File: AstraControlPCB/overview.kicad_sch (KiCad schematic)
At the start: 4 parts

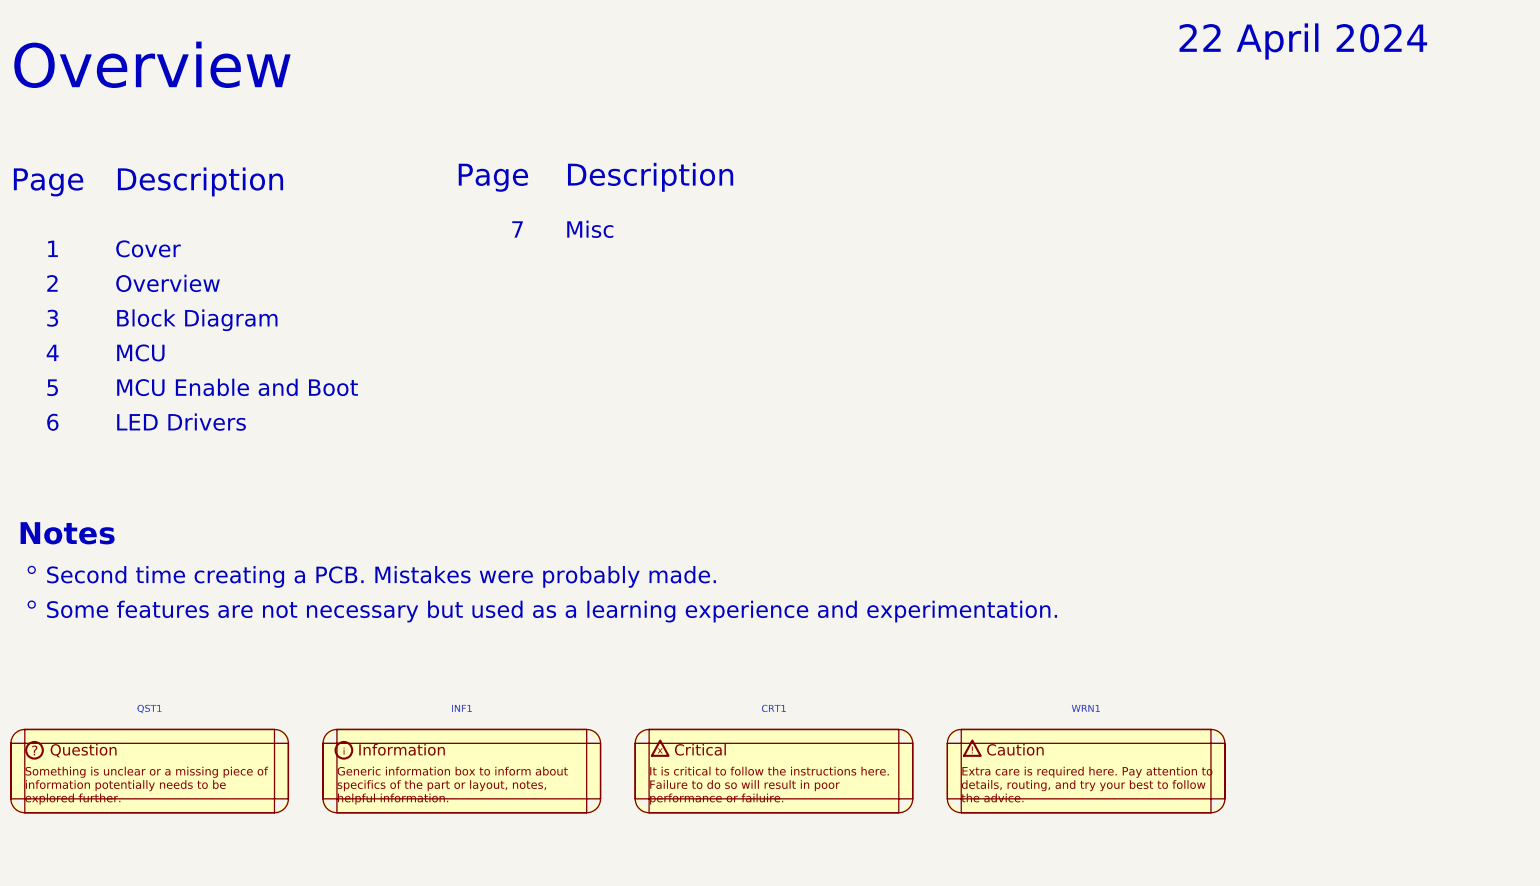
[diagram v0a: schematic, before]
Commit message: update
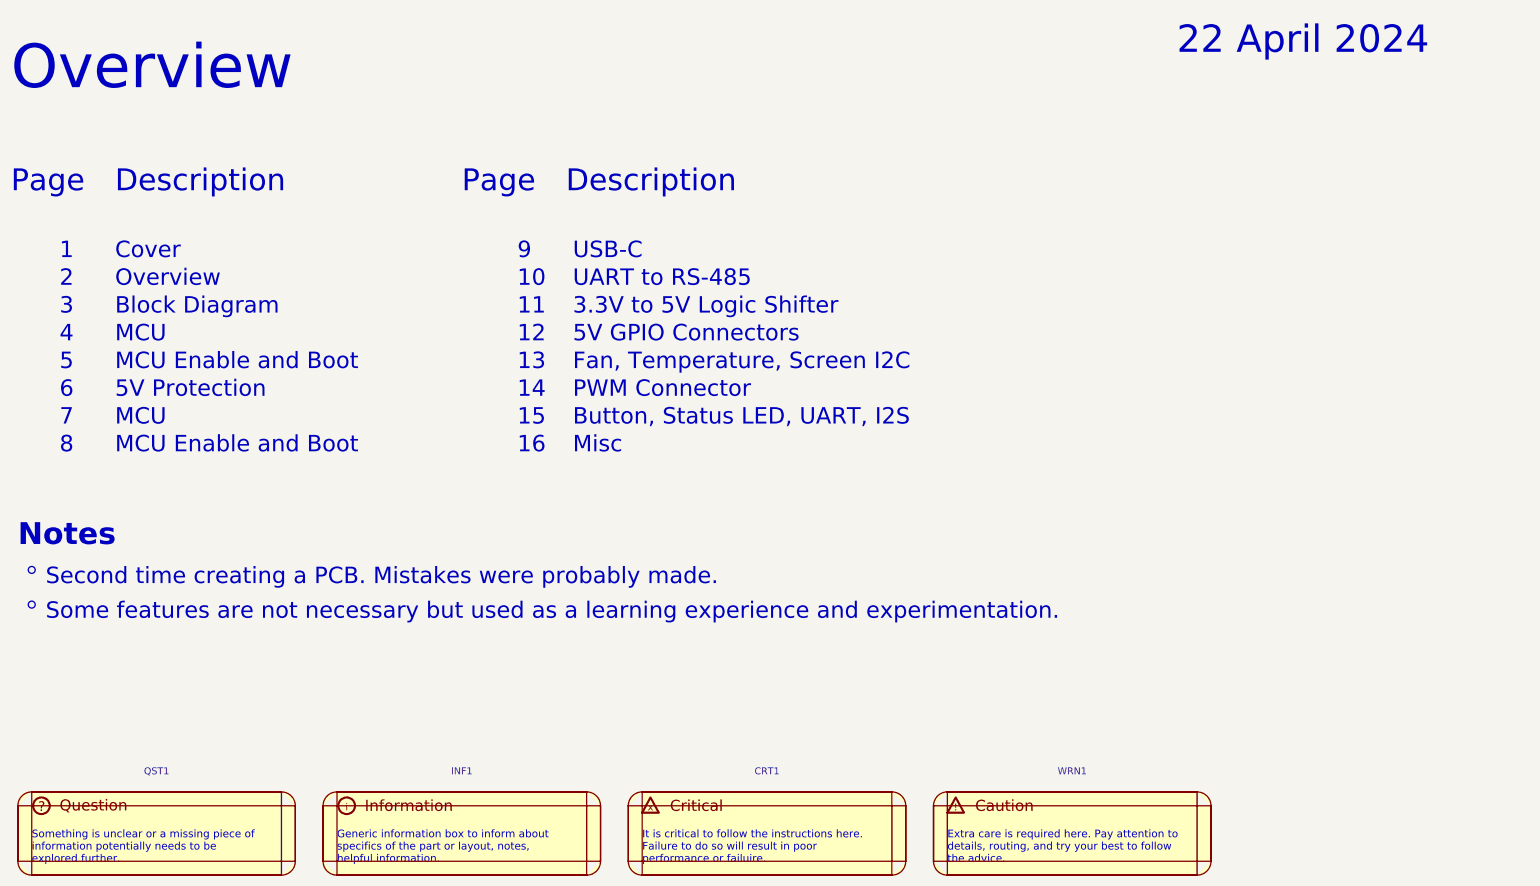
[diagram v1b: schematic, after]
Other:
- note added: "10"
- note added: "11"
- note added: "12"
- note added: "13"
- note added: "14"
- note added: "15"
- note added: "16"
- note added: "3.3V to 5V Logic Shifter"
- note added: "5V GPIO Connectors"
- note added: "5V Protection"
- note added: "8"
- note added: "9"
- note added: "Button, Status LED, UART, I2S"
- note added: "Extra care is required here. Pay attention to details, routing, and try your best to follow the advice."
- note added: "Fan, Temperature, Screen I2C"
- note added: "Generic information box to inform about specifics of the part or layout, notes, helpful information."
- note added: "It is critical to follow the instructions here. Failure to do so will result in poor performance or failuire."
- note added: "PWM Connector"
- note added: "Something is unclear or a missing piece of information potentially needs to be explored further."
- note added: "UART to RS-485"
- note added: "USB-C"
- note removed: "LED Drivers"
